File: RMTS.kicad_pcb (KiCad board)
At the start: 2 copper layers, 45 parts, among them J1 USB_B_Mini, J2 Programmer, J3 Screw_Terminal_01x03, J4 Screw_Terminal_01x04, J5 Screw_Terminal_01x02, J6 Screw_Terminal_01x02, J7 MICRO-SD_CARD_SOCKET, J8 CONN_03, Q1 PMV20ENR, U1 ADP2108AUJ-3.3, U2 MK20DX256VLH7, U3 ADS1219, U4 MCP6N11, Y1 16 Mhz

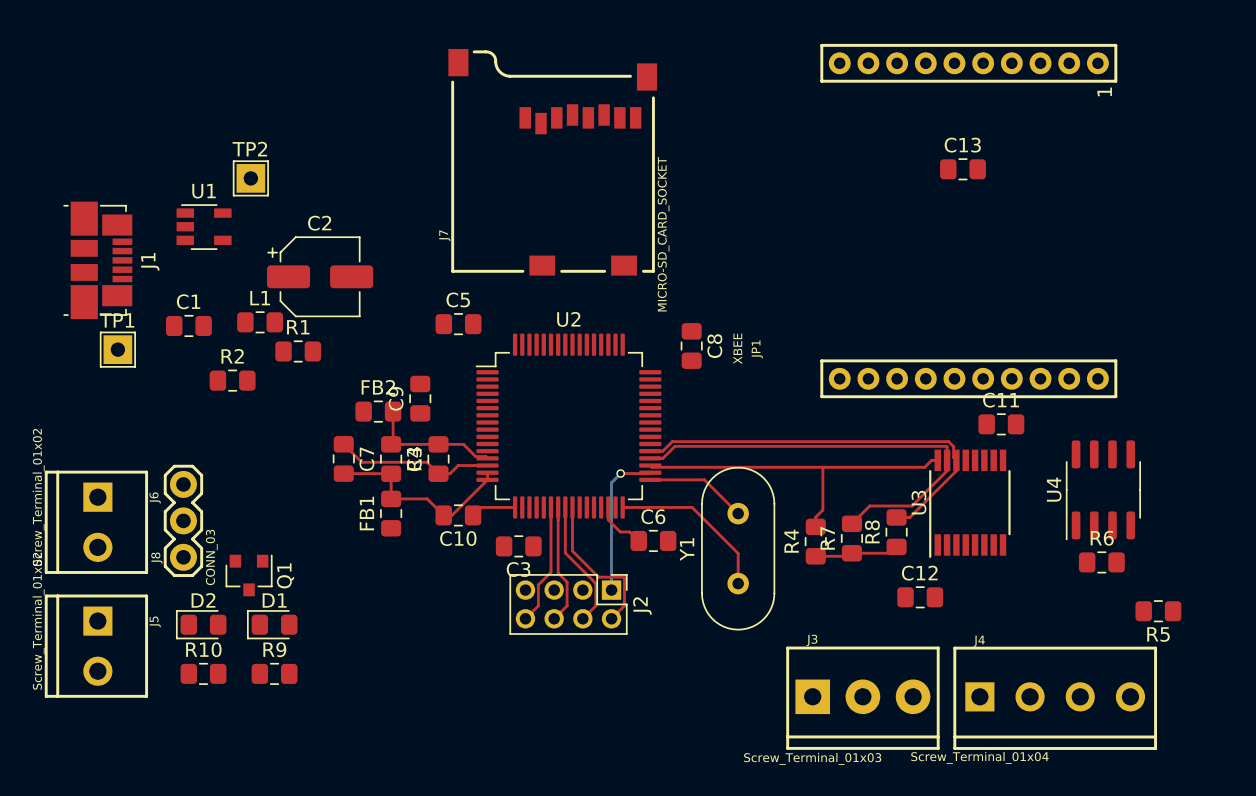
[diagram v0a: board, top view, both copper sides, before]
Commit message: Finished layout
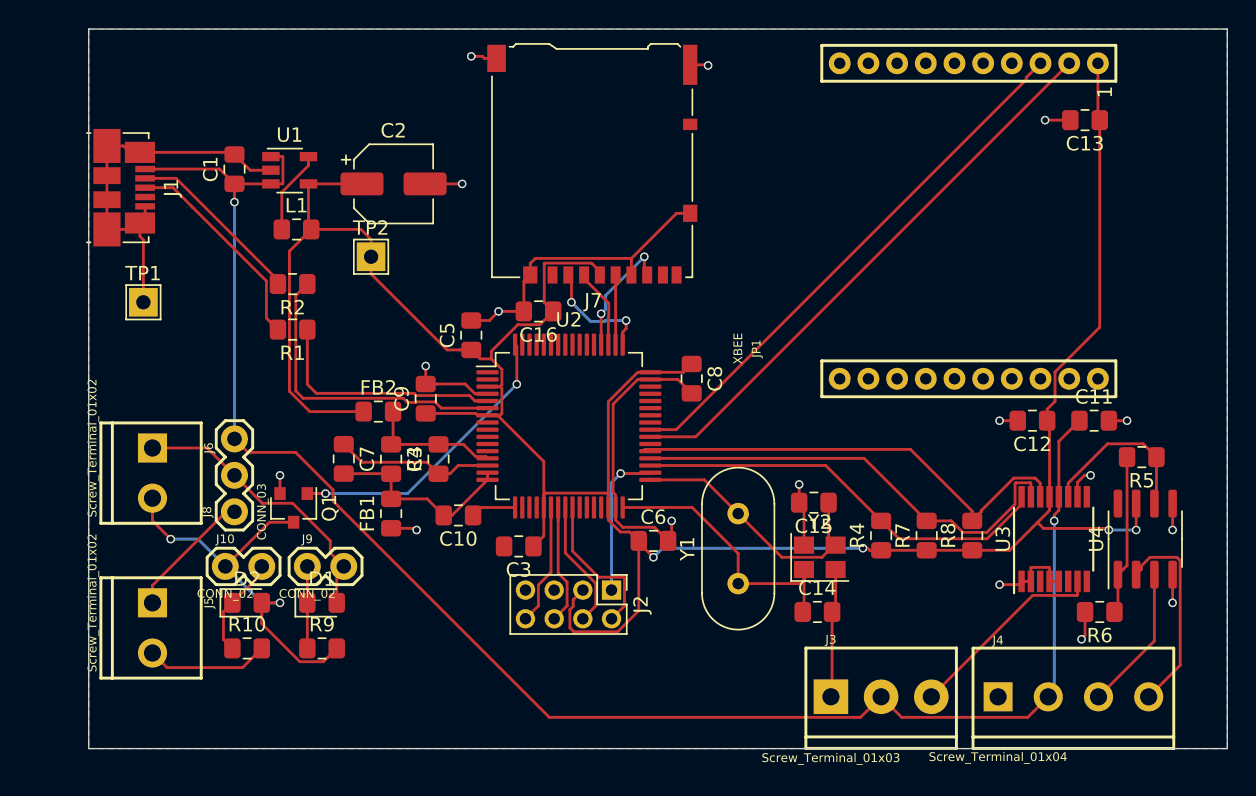
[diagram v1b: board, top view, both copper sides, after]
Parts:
- added C14: 12pF, Capacitor_SMD:C_0805_2012Metric_Pad1.15x1.40mm_HandSolder, F.Cu at (182.9, 102.9)
- added C15: 12pF, Capacitor_SMD:C_0805_2012Metric_Pad1.15x1.40mm_HandSolder, F.Cu at (182.6, 95.2)
- added C16: 0.1uF, Capacitor_SMD:C_0805_2012Metric_Pad1.15x1.40mm_HandSolder, F.Cu at (163.4, 81.9)
- added J10: CONN_02, Connectors:1X02, F.Cu at (141.6, 99.7)
- added J9: CONN_02, Connectors:1X02, F.Cu at (147.3, 99.7)
- added Y2: Crystal_GND24_Small, Crystal:Crystal_SMD_3225-4Pin_3.2x2.5mm, F.Cu at (183.1, 99.1)
- J7: value MICRO-SD_CARD_SOCKET -> Micro_SD_Card_Det_Hirose_DM3AT; footprint Connectors:MICRO-SD-SOCKET -> Connector_Card:microSD_HC_Hirose_DM3AT-SF-PEJM5
- moved C12 14.6 mm to (197.9, 89.5), turned to 180 degrees
- moved C1 11.4 mm to (142.2, 72.0), turned to 90 degrees
- moved R5 10.8 mm to (205.5, 92.1)
- moved TP2 10.0 mm to (151.8, 78.1)
- moved C13 9.17 mm to (201.5, 68.6), turned to 180 degrees
- moved J7 8.60 mm to (167.2, 71.7), turned to 180 degrees
- moved C2 8.26 mm to (153.3, 73.0)
- moved R2 7.92 mm to (146.3, 80.0), turned to 180 degrees
- moved U1 7.15 mm to (146.1, 72.1)
- moved L1 6.96 mm to (146.6, 76.2)
- moved C11 6.47 mm to (202.2, 89.5)
- moved U3 6.37 mm to (199.4, 97.8)
- moved Q1 5.65 mm to (146.4, 95.6)
- moved J1 5.31 mm to (134.6, 73.3)
- moved R8 5.28 mm to (193.7, 97.5)
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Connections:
- net Net-(U2-Pad32) renamed /XTAL1
- net Net-(U2-Pad33) renamed /XTAL2
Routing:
- net +3V3: track 9.50 -> 186.6 mm, vias 0 -> 4
- net GND: track 0.00 -> 124.1 mm, vias 0 -> 17
- net /VBUS: track 0.00 -> 118.0 mm, vias 0 -> 2
- net /DIN: track 0.00 -> 40.0 mm
- net /DOUT: track 0.00 -> 37.9 mm
- net Net-(D2-Pad2): track 0.00 -> 28.3 mm, vias 0 -> 2
- net /USBM: track 0.00 -> 21.7 mm
- net /Fire: track 0.00 -> 20.6 mm, vias 0 -> 2
- net Net-(D1-Pad2): track 0.00 -> 20.0 mm
- net /USBP: track 0.00 -> 16.9 mm
- net Net-(J1-Pad3): track 0.00 -> 15.0 mm
- net Net-(J4-Pad4): track 0.00 -> 14.2 mm
- net Net-(J3-Pad3): track 0.00 -> 14.1 mm
- net Net-(J1-Pad2): track 0.00 -> 12.5 mm
- net /LC0: track 0.00 -> 11.9 mm
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- added copper zone on B.Cu, net GND
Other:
- board outline added: 79.4 x 50.2 mm
